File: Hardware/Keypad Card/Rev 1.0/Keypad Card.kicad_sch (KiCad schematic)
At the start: 11 parts, among them J1 6502 Card Edge, J2 PORT B, J3 PORT A, U1 65C21, U2 AT28C64, U3 74HC138, U4 74HC138

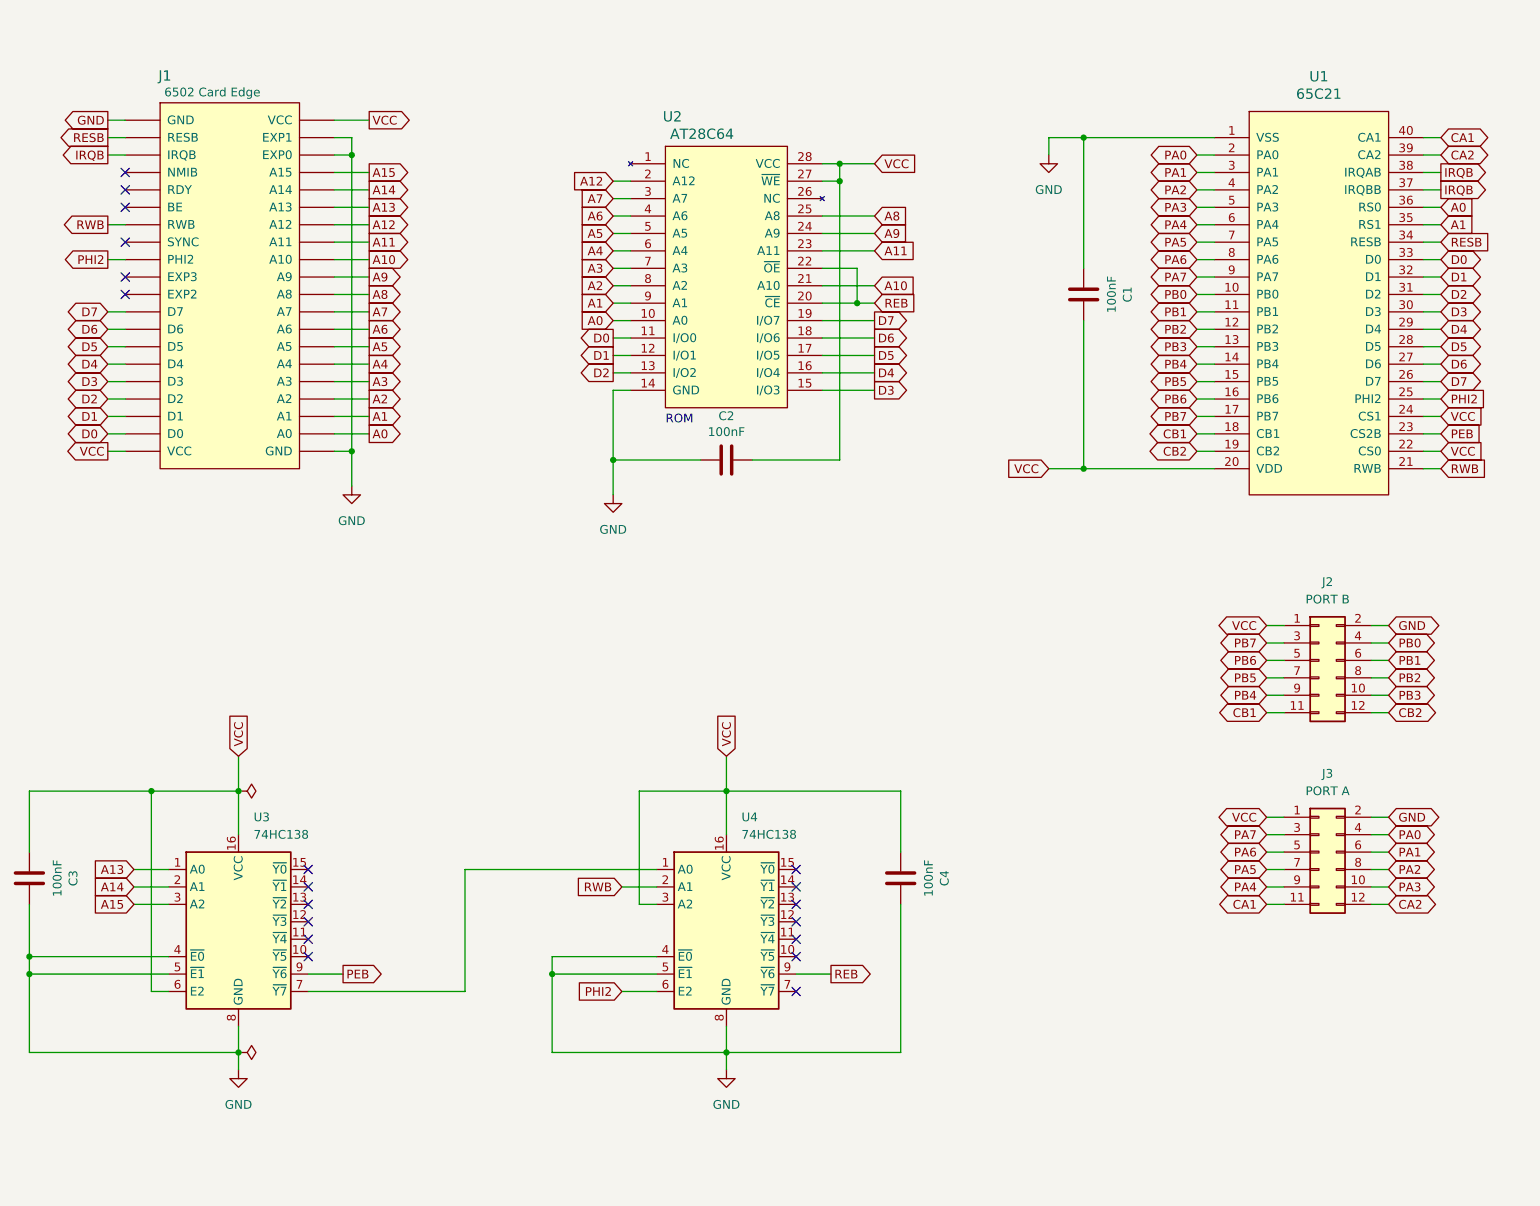
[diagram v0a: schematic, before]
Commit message: Add Keypad Card
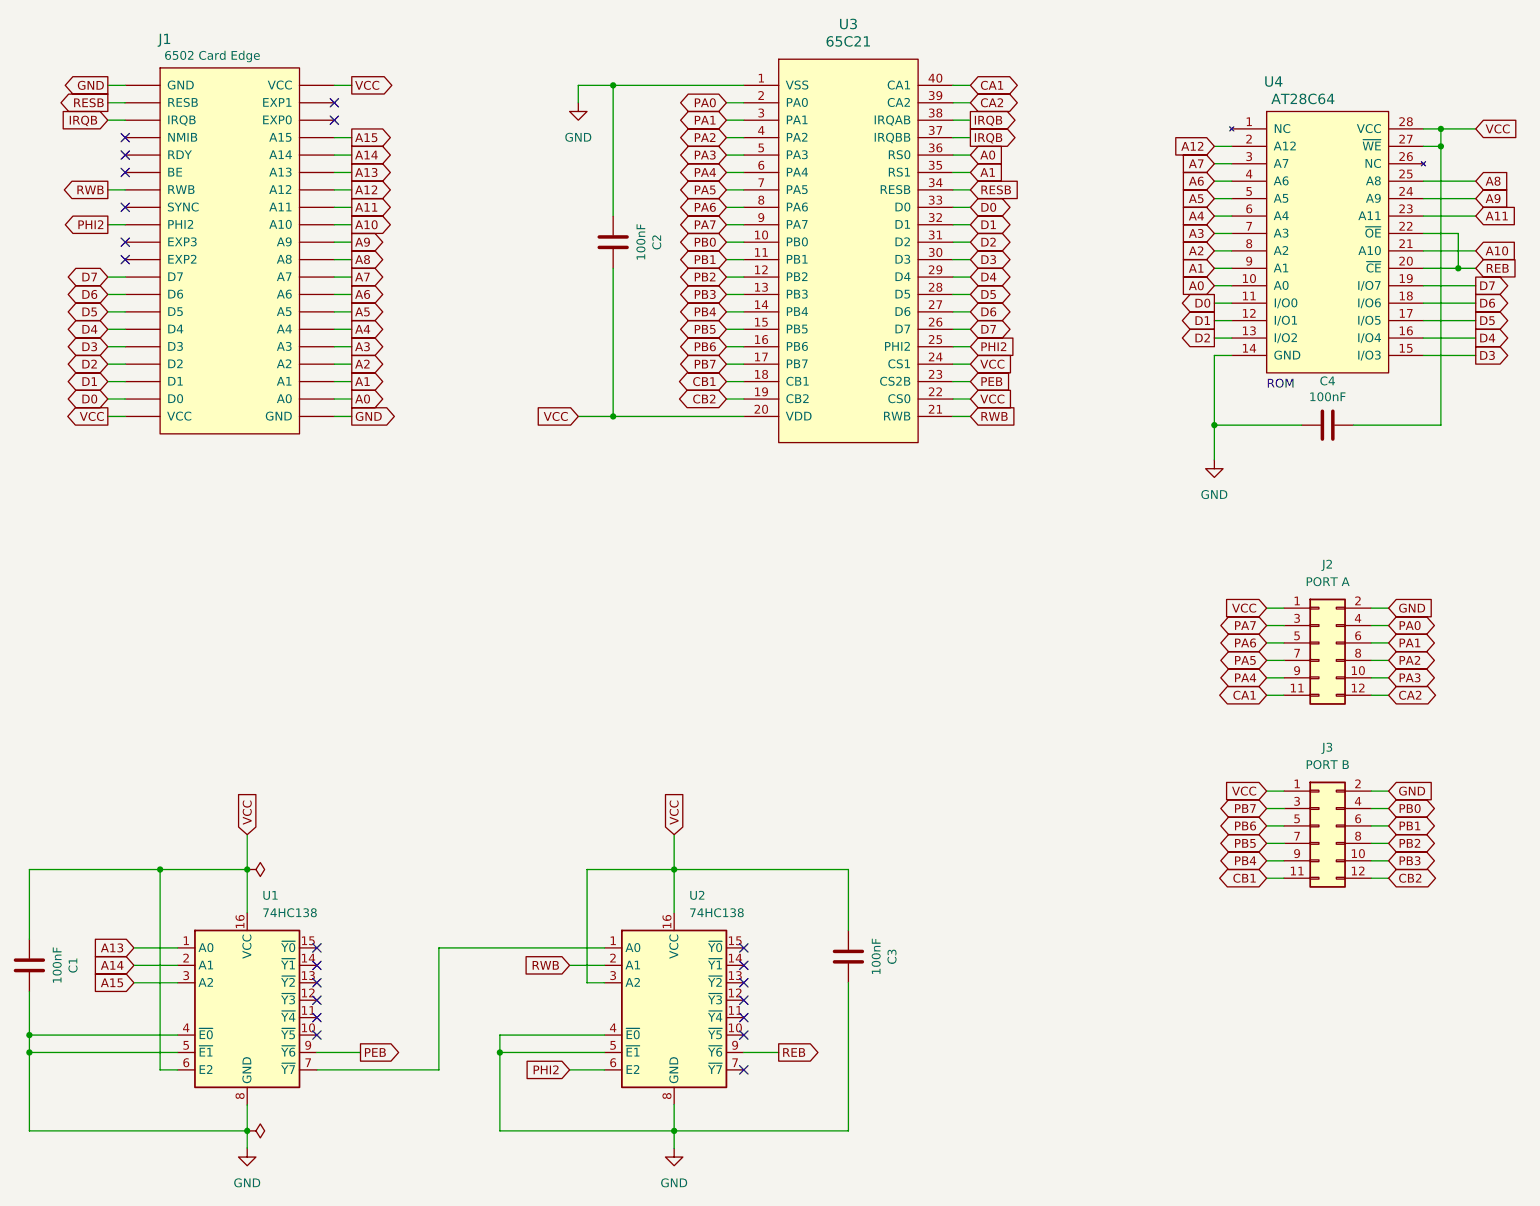
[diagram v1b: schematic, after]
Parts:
- removed U1: 65C21, Package_DIP:DIP-40_W15.24mm_Socket_LongPads, symbol 6502 Parts:65C21
- removed U2: AT28C64, Package_DIP:DIP-28_W15.24mm_Socket_LongPads, symbol 6502 Parts:AT28C64
- removed U4: 74HC138, Package_DIP:DIP-16_W7.62mm_Socket_LongPads, symbol 74xx:74HC138
- added U2: 74HC138, Package_SO:SOIC-16_3.9x9.9mm_P1.27mm, symbol 74xx:74HC138
- added U3: 65C21, Package_DIP:DIP-40_W15.24mm_Socket_LongPads, symbol 6502 Parts:65C21
- added U4: AT28C64, Package_DIP:DIP-28_W15.24mm_Socket_LongPads, symbol 6502 Parts:AT28C64
- C1: footprint Capacitor_THT:C_Disc_D5.0mm_W2.5mm_P5.00mm -> Capacitor_SMD:C_0805_2012Metric
- C2, C3, C4: footprint Capacitor_THT:C_Disc_D5.0mm_W2.5mm_P5.00mm -> Capacitor_SMD:C_0805_2012Metric; LCSC (none) -> C49678
- J2: value PORT B -> PORT A
- J3: value PORT A -> PORT B
- U1: renamed from U3; footprint Package_DIP:DIP-16_W7.62mm_Socket_LongPads -> Package_SO:SOIC-16_3.9x9.9mm_P1.27mm; LCSC (none) -> C5602
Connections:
- net A0: now also U3.36 (RS0), U4.10 (A0)
- net A1: now also U3.35 (RS1), U4.9 (A1)
- net A10: now also U4.21 (A10)
- net A11: now also U4.23 (A11)
- net A12: now also U4.2 (A12)
- net A2: now also U4.8 (A2)
- net A3: now also U4.7 (A3)
- net A4: now also U4.6 (A4)
- net A5: now also U4.5 (A5)
- net A6: now also U4.4 (A6)
- net A7: now also U4.3 (A7)
- net A8: now also U4.25 (A8)
- net A9: now also U4.24 (A9)
- net CA1: now also J2.11 (Pin_11), U3.40 (CA1); no longer J3.11 (Pin_11)
- net CA2: now also J2.12 (Pin_12), U3.39 (CA2); no longer J3.12 (Pin_12)
- net CB1: now also J3.11 (Pin_11), U3.18 (CB1); no longer J2.11 (Pin_11)
- net CB2: now also J3.12 (Pin_12), U3.19 (CB2); no longer J2.12 (Pin_12)
- net D0: now also U3.33 (D0), U4.11 (I/O0)
- net D1: now also U3.32 (D1), U4.12 (I/O1)
- net D2: now also U3.31 (D2), U4.13 (I/O2)
- net D3: now also U3.30 (D3), U4.15 (I/O3)
- net D4: now also U3.29 (D4), U4.16 (I/O4)
- net D5: now also U3.28 (D5), U4.17 (I/O5)
- net D6: now also U3.27 (D6), U4.18 (I/O6)
- net D7: now also U3.26 (D7), U4.19 (I/O7)
- net GND: now also C1.2, C2.1, U2.4 (~{E0}), U2.5 (~{E1}), U2.8 (GND), U3.1 (VSS), U4.14 (GND); no longer C1.1, C2.2, J1.EXP0, J1.EXP1
- net IRQB: now also U3.37 (IRQBB), U3.38 (IRQAB)
- net PA0: now also J2.4 (Pin_4), U3.2 (PA0); no longer J3.4 (Pin_4)
- net PA1: now also J2.6 (Pin_6), U3.3 (PA1); no longer J3.6 (Pin_6)
- net PA2: now also J2.8 (Pin_8), U3.4 (PA2); no longer J3.8 (Pin_8)
- net PA3: now also J2.10 (Pin_10), U3.5 (PA3); no longer J3.10 (Pin_10)
- net PA4: now also J2.9 (Pin_9), U3.6 (PA4); no longer J3.9 (Pin_9)
- net PA5: now also J2.7 (Pin_7), U3.7 (PA5); no longer J3.7 (Pin_7)
- net PA6: now also J2.5 (Pin_5), U3.8 (PA6); no longer J3.5 (Pin_5)
- net PA7: now also J2.3 (Pin_3), U3.9 (PA7); no longer J3.3 (Pin_3)
- net PB0: now also J3.4 (Pin_4), U3.10 (PB0); no longer J2.4 (Pin_4)
- net PB1: now also J3.6 (Pin_6), U3.11 (PB1); no longer J2.6 (Pin_6)
- net PB2: now also J3.8 (Pin_8), U3.12 (PB2); no longer J2.8 (Pin_8)
- net PB3: now also J3.10 (Pin_10), U3.13 (PB3); no longer J2.10 (Pin_10)
- net PB4: now also J3.9 (Pin_9), U3.14 (PB4); no longer J2.9 (Pin_9)
- net PB5: now also J3.7 (Pin_7), U3.15 (PB5); no longer J2.7 (Pin_7)
- net PB6: now also J3.5 (Pin_5), U3.16 (PB6); no longer J2.5 (Pin_5)
- net PB7: now also J3.3 (Pin_3), U3.17 (PB7); no longer J2.3 (Pin_3)
- net PEB: now also U3.23 (CS2B)
- net PHI2: now also U2.6 (E2), U3.25 (PHI2)
- net REB: now also U2.9 (~{Y6}), U4.20 (~{CE}), U4.22 (~{OE})
- net RESB: now also U3.34 (RESB)
- net RWB: now also U2.2 (A1), U3.21 (RWB)
- net VCC: now also C1.1, C2.2, U2.16 (VCC), U2.3 (A2), U3.20 (VDD), U3.22 (CS0), U3.24 (CS1), U4.27 (~{WE}), U4.28 (VCC); no longer C1.2, C2.1
- net at U1.7 (~{Y7}): now also U2.1 (A0)
- no-connect marks 19 -> 21
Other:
- title: 6502 Keypad Expander -> 6502 Keypad Card
- moved on the sheet: U1
